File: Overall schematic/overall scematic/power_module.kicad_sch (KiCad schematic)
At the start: 28 parts, among them IC1 battery protection IC DW01A-G, J1 USB_B_Micro, J2 Conn_01x02_Pin, J3 Conn_01x02_Pin, J4 Conn_01x02_Pin, J5 Conn_01x02_Pin, J6 Conn_01x02_Pin, J7 Battery Charger IC TP4056, Q3 Dual Mosfet FS8205A, U1 MCP1700T-3302E_TT

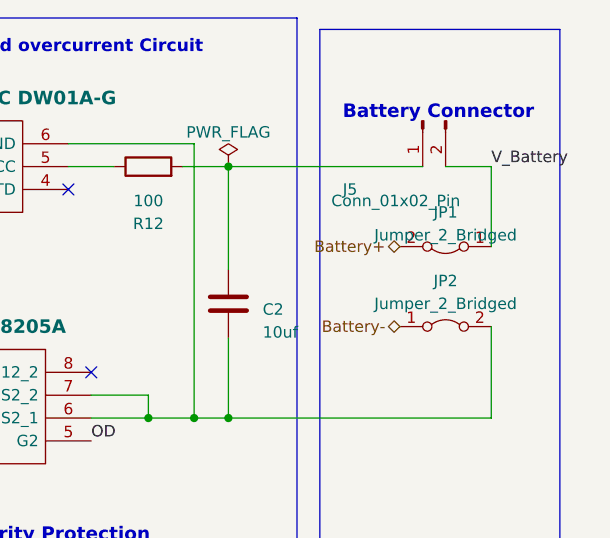
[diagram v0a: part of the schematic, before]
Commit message: the j's
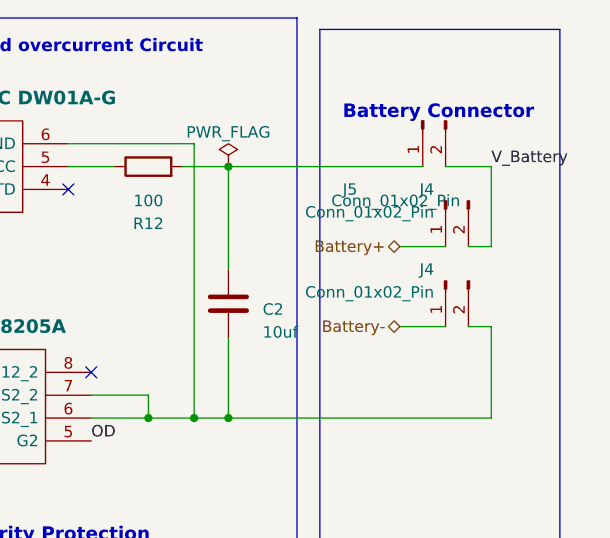
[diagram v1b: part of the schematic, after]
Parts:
- removed JP1, JP2: Jumper_2_Bridged, Jumper:SolderJumper-3_P1.3mm_Bridged12_Pad1.0x1.5mm_NumberLabels, symbol Jumper:Jumper_2_Bridged
- added J4 (x2): Conn_01x02_Pin, Connector_PinHeader_2.54mm:PinHeader_1x02_P2.54mm_Vertical, symbol Connector:Conn_01x02_Pin
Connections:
- net Battery+: now also J4.1 (Pin_1)
- net Battery-: now also J4.1 (Pin_1)
- net V_Battery: now also J4.2 (Pin_2)
- net at C2.2, IC1.6 (GND), Q3.6 (S2_1)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: now also J4.2 (Pin_2)
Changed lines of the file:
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@@
+    (stroke (width 0) (type default))
+  )
+  (wire (pts (xy 262.89 57.15) (xy 267.97 57.15))
     (stroke (width 0) (type default))
   )
@@
     (stroke (width 0) (type default))
   )
+  (wire (pts (xy 270.51 48.26) (xy 273.05 48.26))
+    (stroke (width 0) (type default))
+  )
   (wire (pts (xy 81.28 85.09) (xy 90.17 85.09))
     (stroke (width 0) (type default))
@@
     (stroke (width 0) (type default))
   )
+  (wire (pts (xy 270.51 57.15) (xy 273.05 57.15))
+    (stroke (width 0) (type default))
+  )
   (wire (pts (xy 151.13 64.77) (xy 151.13 69.85))
     (stroke (width 0) (type default))
@@
   )
   (wire (pts (xy 153.67 133.35) (xy 158.75 133.35))
+    (stroke (width 0) (type default))
+  )
+  (wire (pts (xy 262.89 48.26) (xy 267.97 48.26))
     (stroke (width 0) (type default))
   )
@@
         (path "/9230863d-68c5-4e85-a5d4-0f54ecfbae5b/816cf8a9-a5fb-405c-ad63-48cc867f8579"
           (reference "J1") (unit 1)
+        )
+      )
+    )
+  )
+  (symbol (lib_id "Connector:Conn_01x02_Pin") (at 267.97 52.07 90) (mirror x) (unit 1)
+    (in_bom yes) (on_board yes) (dnp no)
+    (property "Reference" "J4" (at 266.7 50.8 90)
+      (effects (font (size 1.27 1.27)) (justify left))
+    )
+    (property "Value" "Conn_01x02_Pin" (at 266.7 53.34 90)
+      (effects (font (size 1.27 1.27)) (justify left))
+    )
+    (property "Footprint" "Connector_PinHeader_2.54mm:PinHeader_1x02_P2.54mm_Vertical" (at 267.97 52.07 0)
+      (effects (font (size 1.27 1.27)) hide)
+    )
+    (property "Datasheet" "https://datasheet.lcsc.com/lcsc/2207291800_ZHOURI-2-54-1-2_C5116481.pdf" (at 267.97 52.07 0)
+      (effects (font (size 1.27 1.27)) hide)
+    )
+    (property "Description" "Plugin,P=2.54mm Pin Headers ROHS" (at 267.97 52.07 0)
+      (effects (font (size 1.27 1.27)) hide)
+    )
+    (property "Manufacturer_Part_Number" "C5116481" (at 267.97 52.07 0)
+      (effects (font (size 1.27 1.27)) hide)
+    )
+    (property "Prices" "$0.0206" (at 267.97 52.07 0)
+      (effects (font (size 1.27 1.27)) hide)
+    )
+    (property "Suppliers" "JLCPCB Parts" (at 267.97 52.07 0)
+      (effects (font (size 1.27 1.27)) hide)
+    )
+    (pin "1")
+    (pin "2")
+    (instances
+      (project "power_module"
+        (path "/1d3f5291-0447-4a85-affa-c96460b342cb"
+          (reference "J4") (unit 1)
+        )
+      )
+      (project "EEE3088F_Schematic"
+        (path "/468ce978-c50a-43bd-b992-da428c4b03d8"
+          (reference "J4") (unit 1)
+        )
+      )
+      (project "overall scematic"
+        (path "/9230863d-68c5-4e85-a5d4-0f54ecfbae5b/816cf8a9-a5fb-405c-ad63-48cc867f8579"
+          (reference "J10") (unit 1)
         )
       )
@@
     )
   )
-  (symbol (lib_id "Jumper:Jumper_2_Bridged") (at 267.97 48.26 180) (unit 1)
-    (in_bom yes) (on_board yes) (dnp no) (fields_autoplaced)
-    (property "Reference" "JP1" (at 267.97 44.45 0)
-      (effects (font (size 1.27 1.27)))
-    )
-    (property "Value" "Jumper_2_Bridged" (at 267.97 46.99 0)
-      (effects (font (size 1.27 1.27)))
-    )
-    (property "Footprint" "Jumper:SolderJumper-3_P1.3mm_Bridged12_Pad1.0x1.5mm_NumberLabels" (at 267.97 48.26 0)
-      (effects (font (size 1.27 1.27)) hide)
-    )
-    (property "Datasheet" "~" (at 267.97 48.26 0)
-      (effects (font (size 1.27 1.27)) hide)
-    )
-    (pin "1")
-    (pin "2")
-    (instances
-      (project "power_module"
-        (path "/1d3f5291-0447-4a85-affa-c96460b342cb"
-          (reference "JP1") (unit 1)
-        )
-      )
-      (project "overall scematic"
-        (path "/9230863d-68c5-4e85-a5d4-0f54ecfbae5b/816cf8a9-a5fb-405c-ad63-48cc867f8579"
-          (reference "JP1") (unit 1)
-        )
-      )
-    )
-  )
   (symbol (lib_id "MCP1700T-3302E_TT:MCP1700T-3302E_TT") (at 135.89 135.89 0) (unit 1)
     (in_bom yes) (on_board yes) (dnp no) (fields_autoplaced)
@@
     )
   )
-  (symbol (lib_id "Jumper:Jumper_2_Bridged") (at 267.97 57.15 0) (unit 1)
-    (in_bom yes) (on_board yes) (dnp no) (fields_autoplaced)
-    (property "Reference" "JP2" (at 267.97 52.07 0)
-      (effects (font (size 1.27 1.27)))
-    )
-    (property "Value" "Jumper_2_Bridged" (at 267.97 54.61 0)
-      (effects (font (size 1.27 1.27)))
-    )
-    (property "Footprint" "Jumper:SolderJumper-3_P1.3mm_Bridged12_Pad1.0x1.5mm_NumberLabels" (at 267.97 57.15 0)
-      (effects (font (size 1.27 1.27)) hide)
-    )
-    (property "Datasheet" "~" (at 267.97 57.15 0)
-      (effects (font (size 1.27 1.27)) hide)
-    )
-    (pin "1")
-    (pin "2")
-    (instances
-      (project "power_module"
-        (path "/1d3f5291-0447-4a85-affa-c96460b342cb"
-          (reference "JP2") (unit 1)
-        )
-      )
-      (project "overall scematic"
-        (path "/9230863d-68c5-4e85-a5d4-0f54ecfbae5b/816cf8a9-a5fb-405c-ad63-48cc867f8579"
-          (reference "JP2") (unit 1)
-        )
-      )
-    )
-  )
   (symbol (lib_id "Connector:Conn_01x02_Pin") (at 176.53 128.27 90) (mirror x) (unit 1)
     (in_bom yes) (on_board yes) (dnp no)
@@
         )
       )
+    )
+  )
+  (symbol (lib_id "Connector:Conn_01x02_Pin") (at 267.97 43.18 90) (mirror x) (unit 1)
+    (in_bom yes) (on_board yes) (dnp no)
+    (property "Reference" "J4" (at 266.7 41.91 90)
+      (effects (font (size 1.27 1.27)) (justify left))
+    )
+    (property "Value" "Conn_01x02_Pin" (at 266.7 44.45 90)
+      (effects (font (size 1.27 1.27)) (justify left))
+    )
+    (property "Footprint" "Connector_PinHeader_2.54mm:PinHeader_1x02_P2.54mm_Vertical" (at 267.97 43.18 0)
+      (effects (font (size 1.27 1.27)) hide)
+    )
+    (property "Datasheet" "https://datasheet.lcsc.com/lcsc/2207291800_ZHOURI-2-54-1-2_C5116481.pdf" (at 267.97 43.18 0)
+      (effects (font (size 1.27 1.27)) hide)
+    )
+    (property "Description" "Plugin,P=2.54mm Pin Headers ROHS" (at 267.97 43.18 0)
+      (effects (font (size 1.27 1.27)) hide)
+    )
+    (property "Manufacturer_Part_Number" "C5116481" (at 267.97 43.18 0)
+      (effects (font (size 1.27 1.27)) hide)
+    )
+    (property "Prices" "$0.0206" (at 267.97 43.18 0)
+      (effects (font (size 1.27 1.27)) hide)
+    )
+    (property "Suppliers" "JLCPCB Parts" (at 267.97 43.18 0)
+      (effects (font (size 1.27 1.27)) hide)
+    )
+    (pin "1")
+    (pin "2")
+    (instances
+      (project "power_module"
+        (path "/1d3f5291-0447-4a85-affa-c96460b342cb"
+          (reference "J4") (unit 1)
+        )
+      )
+      (project "EEE3088F_Schematic"
+        (path "/468ce978-c50a-43bd-b992-da428c4b03d8"
+          (reference "J4") (unit 1)
+        )
+      )
+      (project "overall scematic"
+        (path "/9230863d-68c5-4e85-a5d4-0f54ecfbae5b/816cf8a9-a5fb-405c-ad63-48cc867f8579"
+          (reference "J8") (unit 1)
+        )
+      )
